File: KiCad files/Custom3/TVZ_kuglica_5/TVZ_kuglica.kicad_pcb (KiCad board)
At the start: 2 copper layers, 70 x 80 mm, 36 parts, among them SW1 SW_SPDT

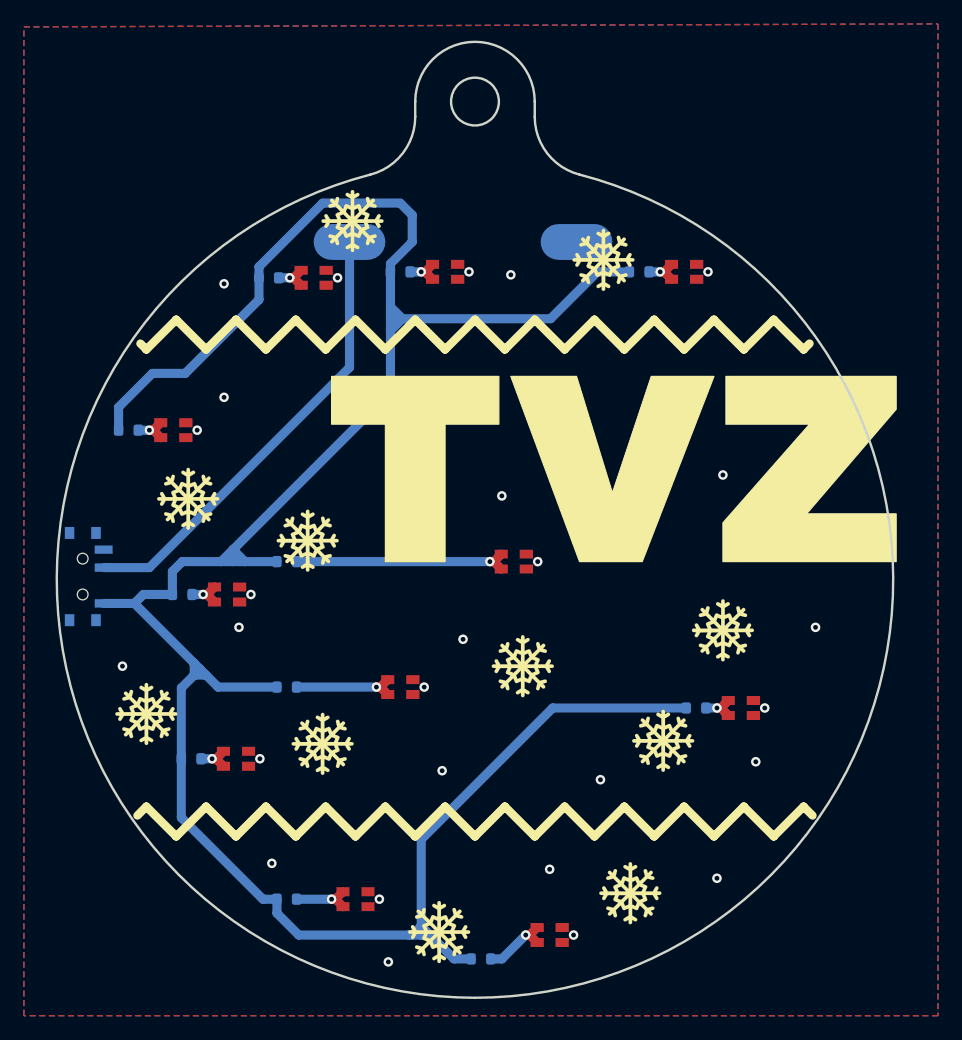
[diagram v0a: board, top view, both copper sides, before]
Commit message: update
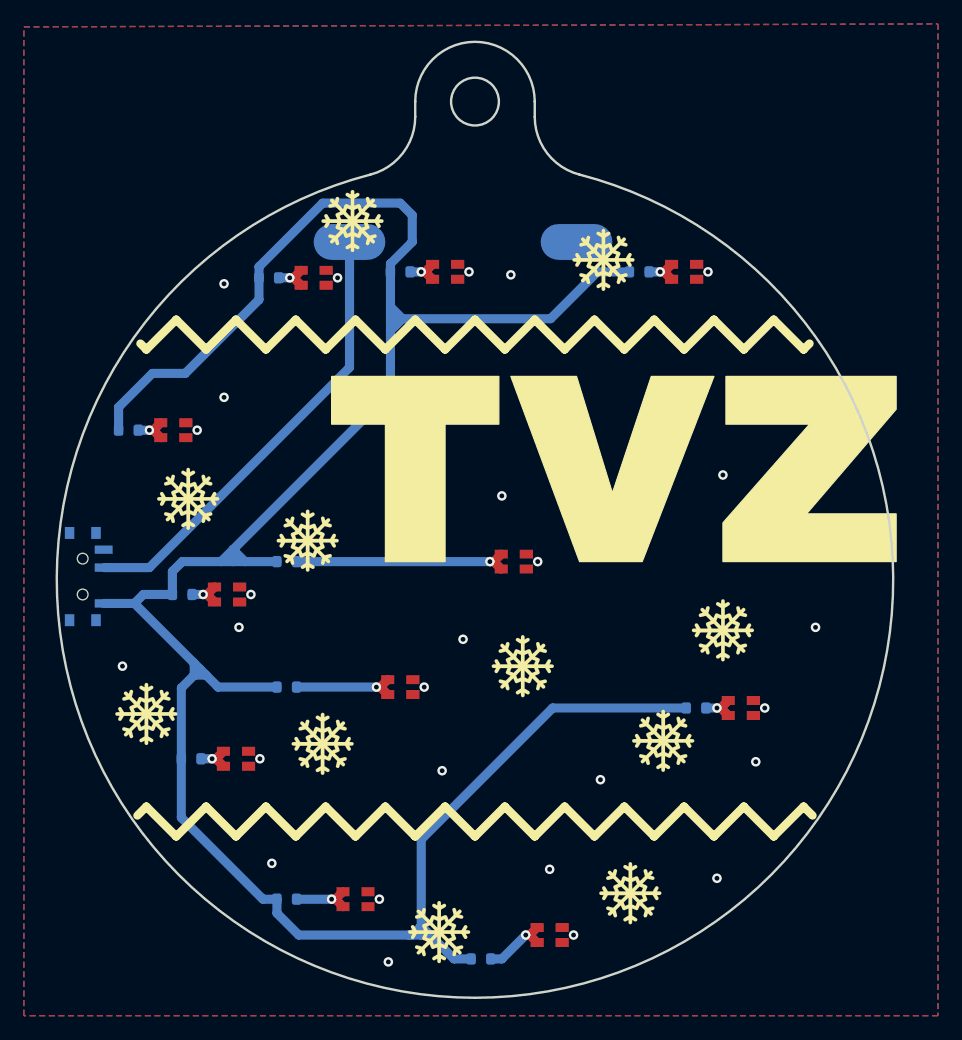
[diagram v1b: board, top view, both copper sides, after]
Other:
- net class Default removed
